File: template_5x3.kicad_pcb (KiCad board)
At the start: 2 copper layers, 0 parts

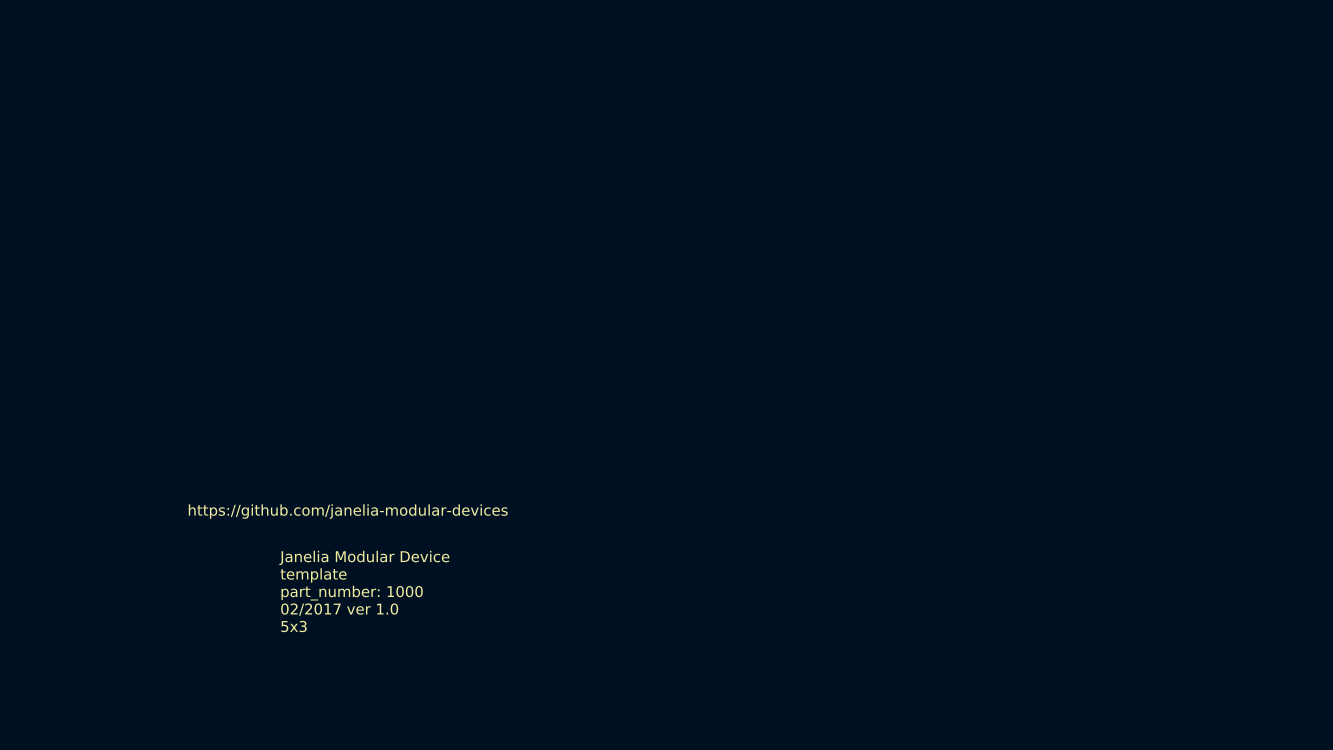
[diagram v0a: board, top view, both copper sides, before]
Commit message: Finished version 1.0.
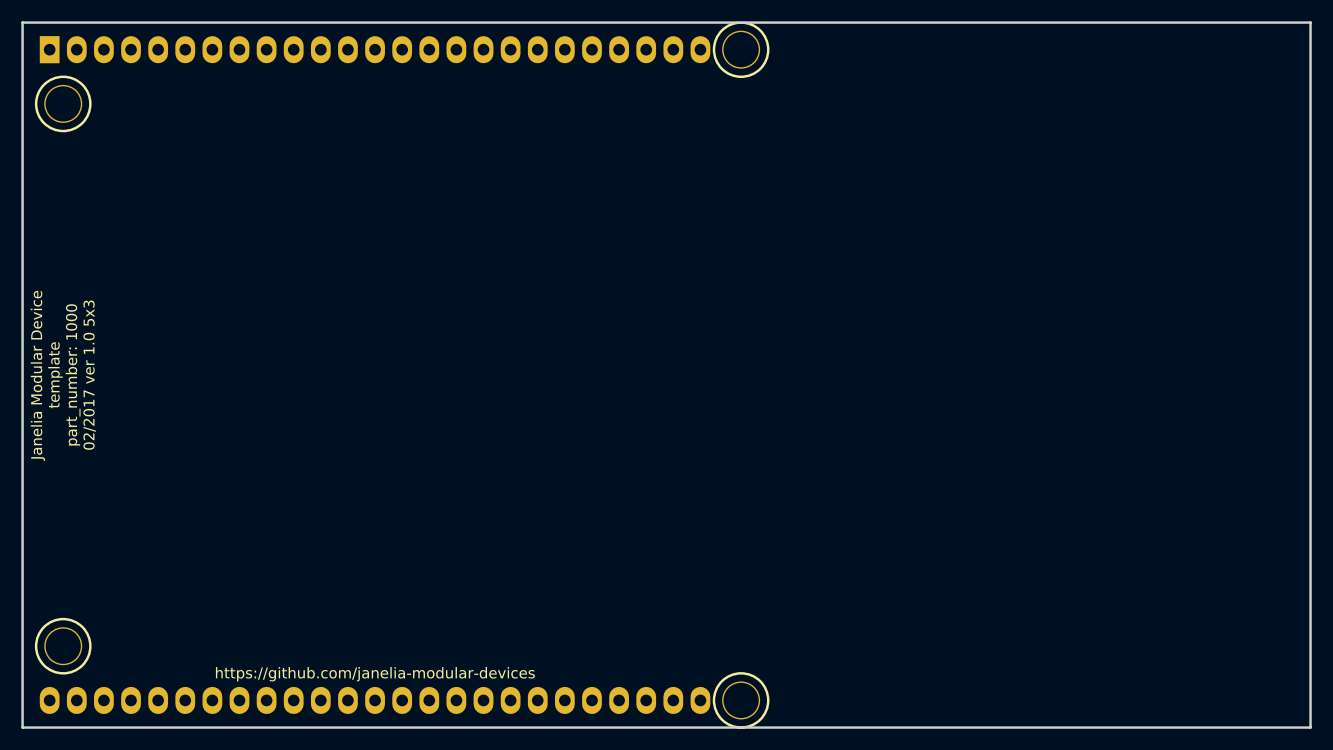
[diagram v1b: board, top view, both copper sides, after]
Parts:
- added MDB1: MODULAR_DEVICE_BASE_5x3_MALE, template_5x3:MODULAR_DEVICE_BASE_5X3_MALE, F.Cu at (91.4, 105.4)
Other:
- board outline added: 120.7 x 66 mm
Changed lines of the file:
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@@
     (links 0)
     (no_connects 0)
-    (area 93.230699 75.196699 211.569301 130.543301)
+    (area 0 0 0 0)
     (thickness 1.6)
-    (drawings 2)
+    (drawings 6)
     (tracks 0)
     (zones 0)
-    (modules 0)
+    (modules 1)
     (nets 1)
   )
@@
     (diff_pair_width 0.254)
   )
-  (gr_text https://github.com/janelia-modular-devices (at 100.33 118.11) (layer F.SilkS)
+  (module template_5x3:MODULAR_DEVICE_BASE_5X3_MALE (layer F.Cu)
+    (at 91.44 105.41)
+    (fp_text reference MDB1 (at 0 0) (layer F.SilkS) hide
+      (effects (font (size 1.016 1.016) (thickness 0.254)))
+    )
+    (fp_text value MODULAR_DEVICE_BASE_5x3_MALE (at 0 2.54) (layer F.SilkS) hide
+      (effects (font (thickness 0.3048)))
+    )
+    (fp_line (start -20.32 29.21) (end -20.32 31.75) (layer B.SilkS) (width 0.381))
+    (fp_line (start 43.18 31.75) (end 43.18 29.21) (layer B.SilkS) (width 0.381))
+    (fp_line (start -20.32 -31.75) (end -20.32 -29.21) (layer B.SilkS) (width 0.381))
+    (fp_line (start 43.18 -29.21) (end 43.18 -31.75) (layer B.SilkS) (width 0.381))
+    (fp_line (start -21.59 -33.02) (end -21.59 33.02) (layer F.Fab) (width 0.2286))
+    (fp_line (start -21.59 33.02) (end 99.06 33.02) (layer F.Fab) (width 0.2286))
+    (fp_line (start 99.06 33.02) (end 99.06 -33.02) (layer F.Fab) (width 0.2286))
+    (fp_line (start 99.06 -33.02) (end -21.59 -33.02) (layer F.Fab) (width 0.2286))
+    (fp_line (start -20.32 29.21) (end 43.18 29.21) (layer B.SilkS) (width 0.381))
+    (fp_line (start -20.32 31.75) (end 43.18 31.75) (layer B.SilkS) (width 0.381))
+    (fp_line (start -20.32 -31.75) (end 43.18 -31.75) (layer B.SilkS) (width 0.381))
+    (fp_line (start -20.32 -29.21) (end 43.18 -29.21) (layer B.SilkS) (width 0.381))
+    (fp_circle (center -17.78 -25.4) (end -15.24 -25.4) (layer F.SilkS) (width 0.2286))
+    (fp_circle (center -17.78 25.4) (end -15.24 25.4) (layer F.SilkS) (width 0.2286))
+    (fp_circle (center 45.72 -30.48) (end 48.26 -30.48) (layer F.SilkS) (width 0.2286))
+    (fp_circle (center 45.72 30.48) (end 48.26 30.48) (layer F.SilkS) (width 0.2286))
+    (pad GND thru_hole oval (at -16.51 -30.48) (size 1.8542 2.54) (drill 1.0922) (layers *.Cu *.Mask))
+    (pad A10 thru_hole oval (at -13.97 -30.48) (size 1.8542 2.54) (drill 1.0922) (layers *.Cu *.Mask))
+    (pad VDD thru_hole rect (at -19.05 -30.48) (size 1.8542 2.54) (drill 1.0922) (layers *.Cu *.Mask))
+    (pad A11 thru_hole oval (at -11.43 -30.48) (size 1.8542 2.54) (drill 1.0922) (layers *.Cu *.Mask))
+    (pad 2 thru_hole oval (at -8.89 -30.48) (size 1.8542 2.54) (drill 1.0922) (layers *.Cu *.Mask))
+    (pad 55 thru_hole oval (at -6.35 -30.48) (size 1.8542 2.54) (drill 1.0922) (layers *.Cu *.Mask))
+    (pad 54 thru_hole oval (at -3.81 -30.48) (size 1.8542 2.54) (drill 1.0922) (layers *.Cu *.Mask))
+    (pad 5 thru_hole oval (at -1.27 -30.48) (size 1.8542 2.54) (drill 1.0922) (layers *.Cu *.Mask))
+    (pad 6 thru_hole oval (at 1.27 -30.48) (size 1.8542 2.54) (drill 1.0922) (layers *.Cu *.Mask))
+    (pad 52 thru_hole oval (at 3.81 -30.48) (size 1.8542 2.54) (drill 1.0922) (layers *.Cu *.Mask))
+    (pad 40 thru_hole oval (at 6.35 -30.48) (size 1.8542 2.54) (drill 1.0922) (layers *.Cu *.Mask))
+    (pad 41 thru_hole oval (at 8.89 -30.48) (size 1.8542 2.54) (drill 1.0922) (layers *.Cu *.Mask))
+    (pad 42 thru_hole oval (at 11.43 -30.48) (size 1.8542 2.54) (drill 1.0922) (layers *.Cu *.Mask))
+    (pad 11 thru_hole oval (at 13.97 -30.48) (size 1.8542 2.54) (drill 1.0922) (layers *.Cu *.Mask))
+    (pad 12 thru_hole oval (at 16.51 -30.48) (size 1.8542 2.54) (drill 1.0922) (layers *.Cu *.Mask))
+    (pad 50 thru_hole oval (at 19.05 -30.48) (size 1.8542 2.54) (drill 1.0922) (layers *.Cu *.Mask))
+    (pad 53 thru_hole oval (at 19.05 30.48) (size 1.8542 2.54) (drill 1.0922) (layers *.Cu *.Mask))
+    (pad 13 thru_hole oval (at 16.51 30.48) (size 1.8542 2.54) (drill 1.0922) (layers *.Cu *.Mask))
+    (pad 14 thru_hole oval (at 13.97 30.48) (size 1.8542 2.54) (drill 1.0922) (layers *.Cu *.Mask))
+    (pad 15 thru_hole oval (at 11.43 30.48) (size 1.8542 2.54) (drill 1.0922) (layers *.Cu *.Mask))
+    (pad 16 thru_hole oval (at 8.89 30.48) (size 1.8542 2.54) (drill 1.0922) (layers *.Cu *.Mask))
+    (pad 17 thru_hole oval (at 6.35 30.48) (size 1.8542 2.54) (drill 1.0922) (layers *.Cu *.Mask))
+    (pad 18 thru_hole oval (at 3.81 30.48) (size 1.8542 2.54) (drill 1.0922) (layers *.Cu *.Mask))
+    (pad 19 thru_hole oval (at 1.27 30.48) (size 1.8542 2.54) (drill 1.0922) (layers *.Cu *.Mask))
+    (pad 20 thru_hole oval (at -1.27 30.48) (size 1.8542 2.54) (drill 1.0922) (layers *.Cu *.Mask))
+    (pad 21 thru_hole oval (at -3.81 30.48) (size 1.8542 2.54) (drill 1.0922) (layers *.Cu *.Mask))
+    (pad 22 thru_hole oval (at -6.35 30.48) (size 1.8542 2.54) (drill 1.0922) (layers *.Cu *.Mask))
+    (pad 23 thru_hole oval (at -8.89 30.48) (size 1.8542 2.54) (drill 1.0922) (layers *.Cu *.Mask))
+    (pad 3V3 thru_hole oval (at -11.43 30.48) (size 1.8542 2.54) (drill 1.0922) (layers *.Cu *.Mask))
+    (pad AGND thru_hole oval (at -13.97 30.48) (size 1.8542 2.54) (drill 1.0922) (layers *.Cu *.Mask))
+    (pad VEE thru_hole oval (at -16.51 30.48) (size 1.8542 2.54) (drill 1.0922) (layers *.Cu *.Mask))
+    (pad AREF thru_hole oval (at -19.05 30.48) (size 1.8542 2.54) (drill 1.0922) (layers *.Cu *.Mask))
+    (pad "" thru_hole circle (at -17.78 -25.4) (size 3.556 3.556) (drill 3.302) (layers *.Cu *.Mask F.SilkS))
+    (pad "" thru_hole circle (at -17.78 25.4) (size 3.556 3.556) (drill 3.302) (layers *.Cu *.Mask F.SilkS))
+    (pad "" thru_hole circle (at 45.72 30.48) (size 3.556 3.556) (drill 3.302) (layers *.Cu *.Mask F.SilkS))
+    (pad "" thru_hole circle (at 45.72 -30.48) (size 3.556 3.556) (drill 3.302) (layers *.Cu *.Mask F.SilkS))
+    (pad DAC1 thru_hole oval (at 21.59 30.48) (size 1.8542 2.54) (drill 1.0922) (layers *.Cu *.Mask))
+    (pad DAC0 thru_hole oval (at 24.13 30.48) (size 1.8542 2.54) (drill 1.0922) (layers *.Cu *.Mask))
+    (pad 51 thru_hole oval (at 26.67 30.48) (size 1.8542 2.54) (drill 1.0922) (layers *.Cu *.Mask))
+    (pad 38 thru_hole oval (at 29.21 30.48) (size 1.8542 2.54) (drill 1.0922) (layers *.Cu *.Mask))
+    (pad 37 thru_hole oval (at 31.75 30.48) (size 1.8542 2.54) (drill 1.0922) (layers *.Cu *.Mask))
+    (pad 36 thru_hole oval (at 34.29 30.48) (size 1.8542 2.54) (drill 1.0922) (layers *.Cu *.Mask))
+    (pad 35 thru_hole oval (at 36.83 30.48) (size 1.8542 2.54) (drill 1.0922) (layers *.Cu *.Mask))
+    (pad 34 thru_hole oval (at 39.37 30.48) (size 1.8542 2.54) (drill 1.0922) (layers *.Cu *.Mask))
+    (pad 33 thru_hole oval (at 41.91 30.48) (size 1.8542 2.54) (drill 1.0922) (layers *.Cu *.Mask))
+    (pad 49 thru_hole oval (at 21.59 -30.48) (size 1.8542 2.54) (drill 1.0922) (layers *.Cu *.Mask))
+    (pad 48 thru_hole oval (at 24.13 -30.48) (size 1.8542 2.54) (drill 1.0922) (layers *.Cu *.Mask))
+    (pad 47 thru_hole oval (at 26.67 -30.48) (size 1.8542 2.54) (drill 1.0922) (layers *.Cu *.Mask))
+    (pad 43 thru_hole oval (at 29.21 -30.48) (size 1.8542 2.54) (drill 1.0922) (layers *.Cu *.Mask))
+    (pad 44 thru_hole oval (at 31.75 -30.48) (size 1.8542 2.54) (drill 1.0922) (layers *.Cu *.Mask))
+    (pad 29 thru_hole oval (at 34.29 -30.48) (size 1.8542 2.54) (drill 1.0922) (layers *.Cu *.Mask))
+    (pad 30 thru_hole oval (at 36.83 -30.48) (size 1.8542 2.54) (drill 1.0922) (layers *.Cu *.Mask))
+    (pad 45 thru_hole oval (at 39.37 -30.48) (size 1.8542 2.54) (drill 1.0922) (layers *.Cu *.Mask))
+    (pad 46 thru_hole oval (at 41.91 -30.48) (size 1.8542 2.54) (drill 1.0922) (layers *.Cu *.Mask))
+  )
+  (gr_line (start 190.5 72.39) (end 69.85 72.39) (angle 90) (layer Edge.Cuts) (width 0.2286))
+  (gr_line (start 190.5 138.43) (end 190.5 72.39) (angle 90) (layer Edge.Cuts) (width 0.2286))
+  (gr_line (start 69.85 138.43) (end 190.5 138.43) (angle 90) (layer Edge.Cuts) (width 0.2286))
+  (gr_line (start 69.85 72.39) (end 69.85 138.43) (angle 90) (layer Edge.Cuts) (width 0.2286))
+  (gr_text https://github.com/janelia-modular-devices (at 102.87 133.35) (layer F.SilkS)
     (effects (font (size 1.016 1.016) (thickness 0.1905)))
   )
-  (gr_text "Janelia Modular Device\ntemplate\npart_number: 1000\n02/2017 ver 1.0\n5x3" (at 93.98 125.73) (layer F.SilkS)
-    (effects (font (size 1.016 1.016) (thickness 0.254)) (justify left))
+  (gr_text "Janelia Modular Device\ntemplate\npart_number: 1000\n02/2017 ver 1.0 5x3" (at 73.66 105.41 90) (layer F.SilkS)
+    (effects (font (size 1.016 1.016) (thickness 0.254)))
   )
 )
